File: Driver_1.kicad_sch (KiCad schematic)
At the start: 36 parts

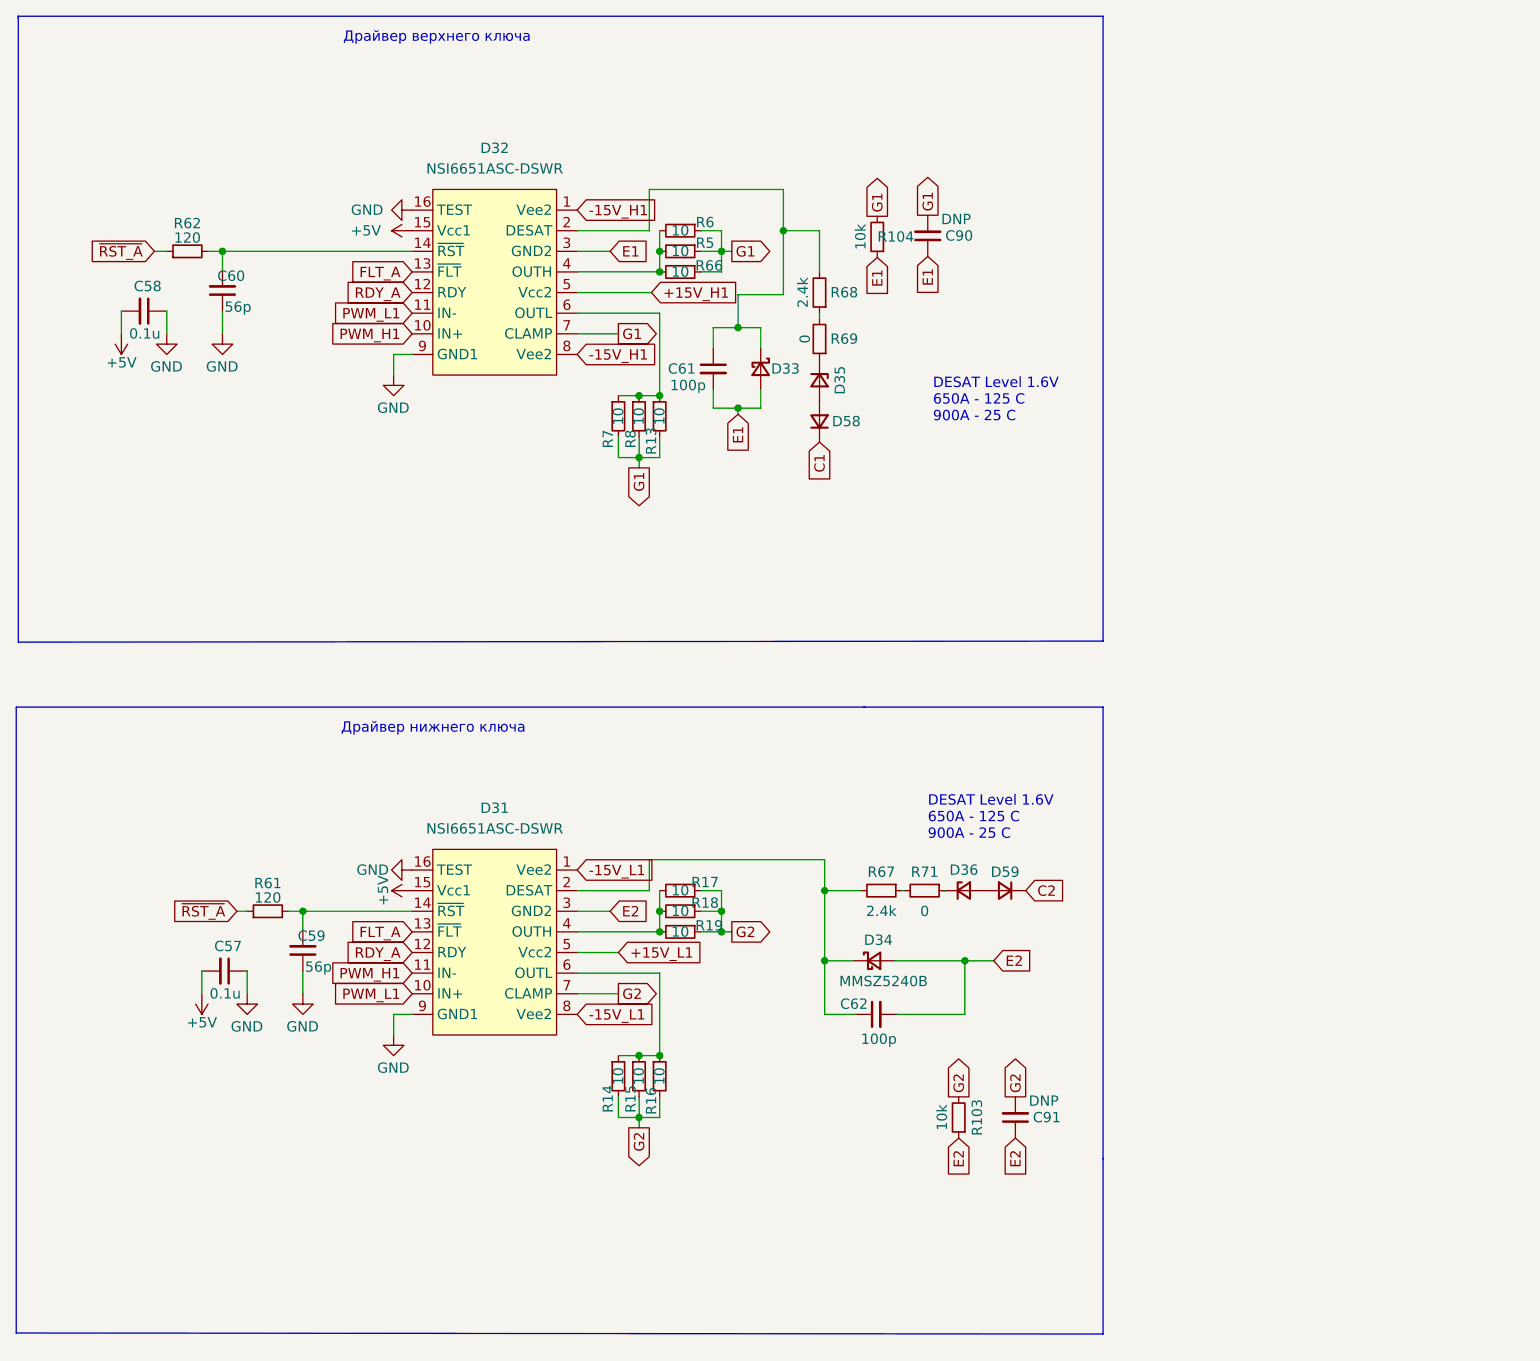
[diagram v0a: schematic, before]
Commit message: VER2.1: добавил СБ и 3D модели в доки
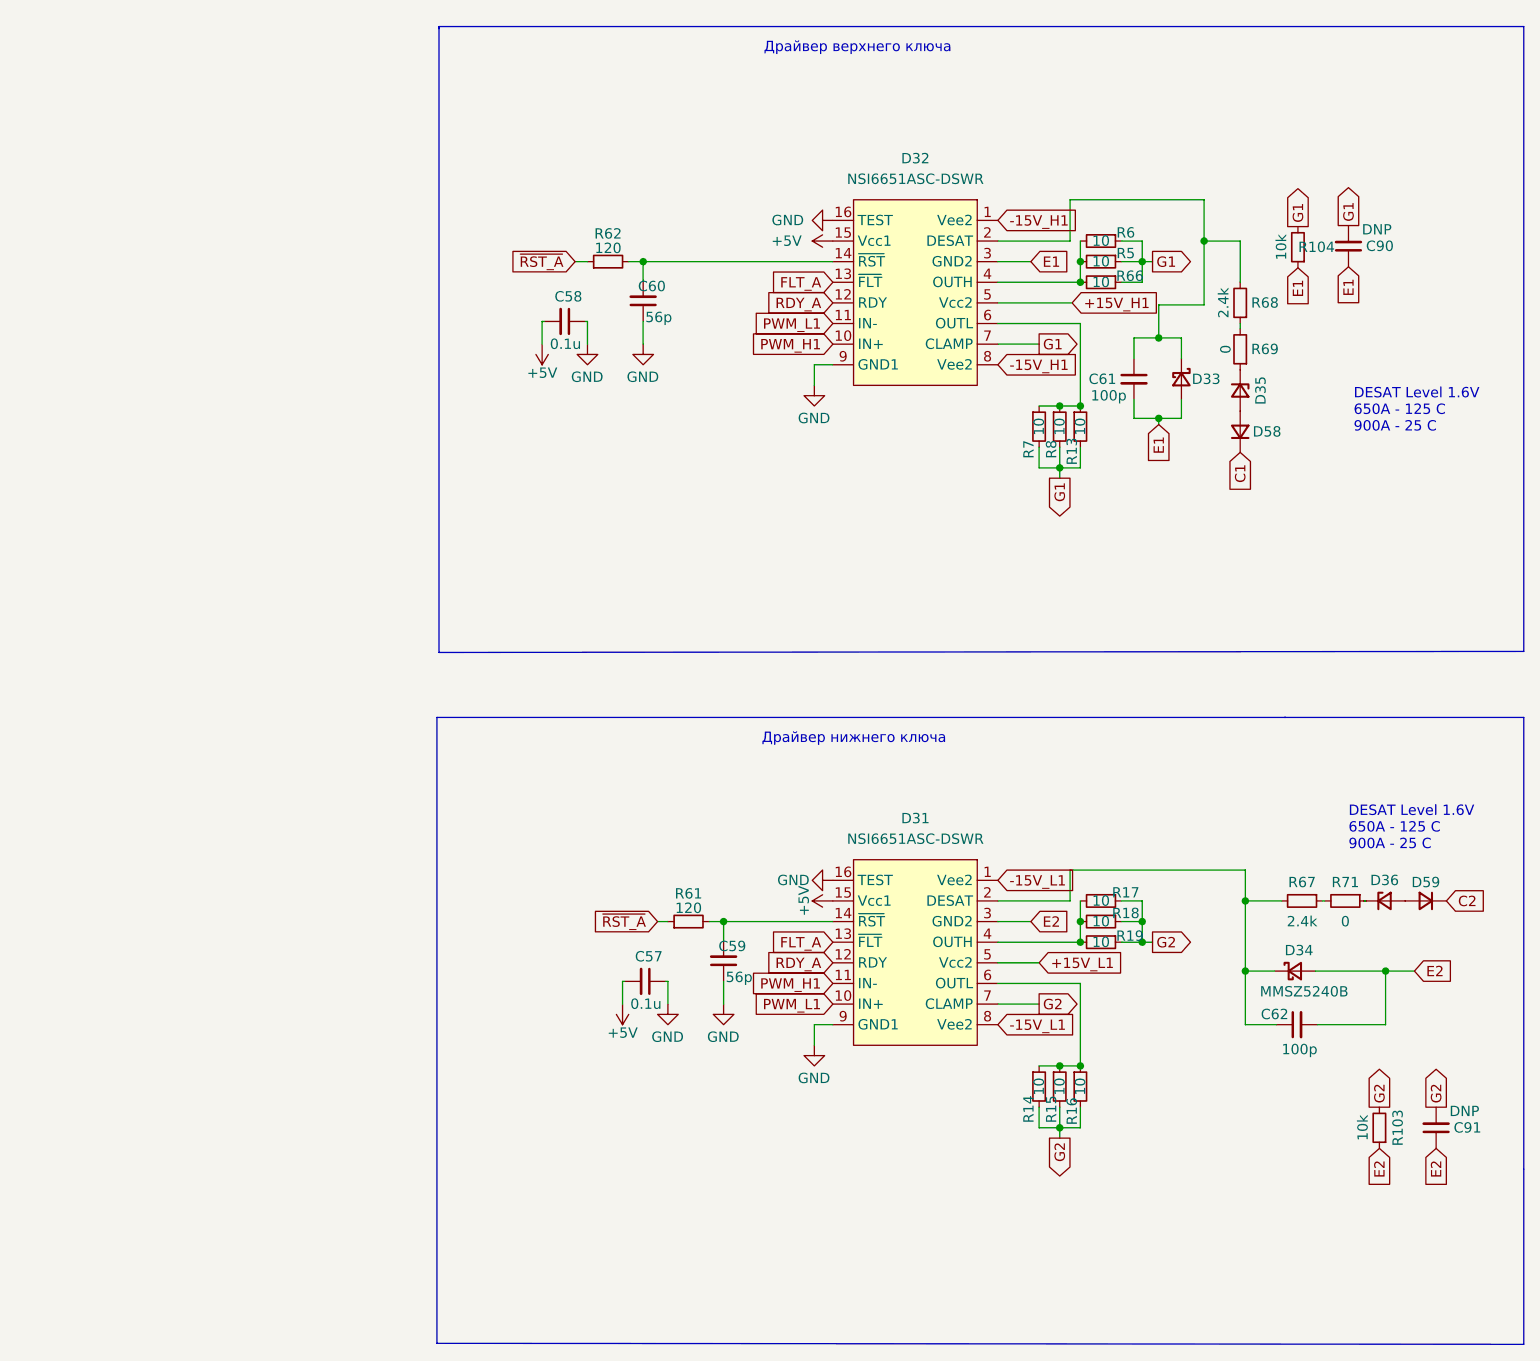
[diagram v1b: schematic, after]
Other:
- moved on the sheet: C57, C58, C59, C60, C61, C62, C90, C91, D31, D32, D33, D34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
